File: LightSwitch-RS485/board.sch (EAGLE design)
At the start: 86 parts, among them IC1 PCF8574T, IC2 PCF8574T, K1 OMRON-G3MB-202P-SSR, K2 OMRON-G3MB-202P-SSR, K20 691218410003, K21 691218410003, K22 691218410003, K3 OMRON-G3MB-202P-SSR, K4 OMRON-G3MB-202P-SSR, K5 OMRON-G3MB-202P-SSR, K6 OMRON-G3MB-202P-SSR, K7 OMRON-G3MB-202P-SSR, K8 OMRON-G3MB-202P-SSR, K9 691218410003, T1 BC847, T2 BC847, T3 BC847, T4 BC847, T5 BC847, T6 BC847, T7 BC847, T8 BC847, U1 MAX487ESA+TCBX, U2 ATMEGA328, X1 JST-XH-04-PIN-LONG-PAD, X2 JST-XH-09-PIN-LONG-PAD

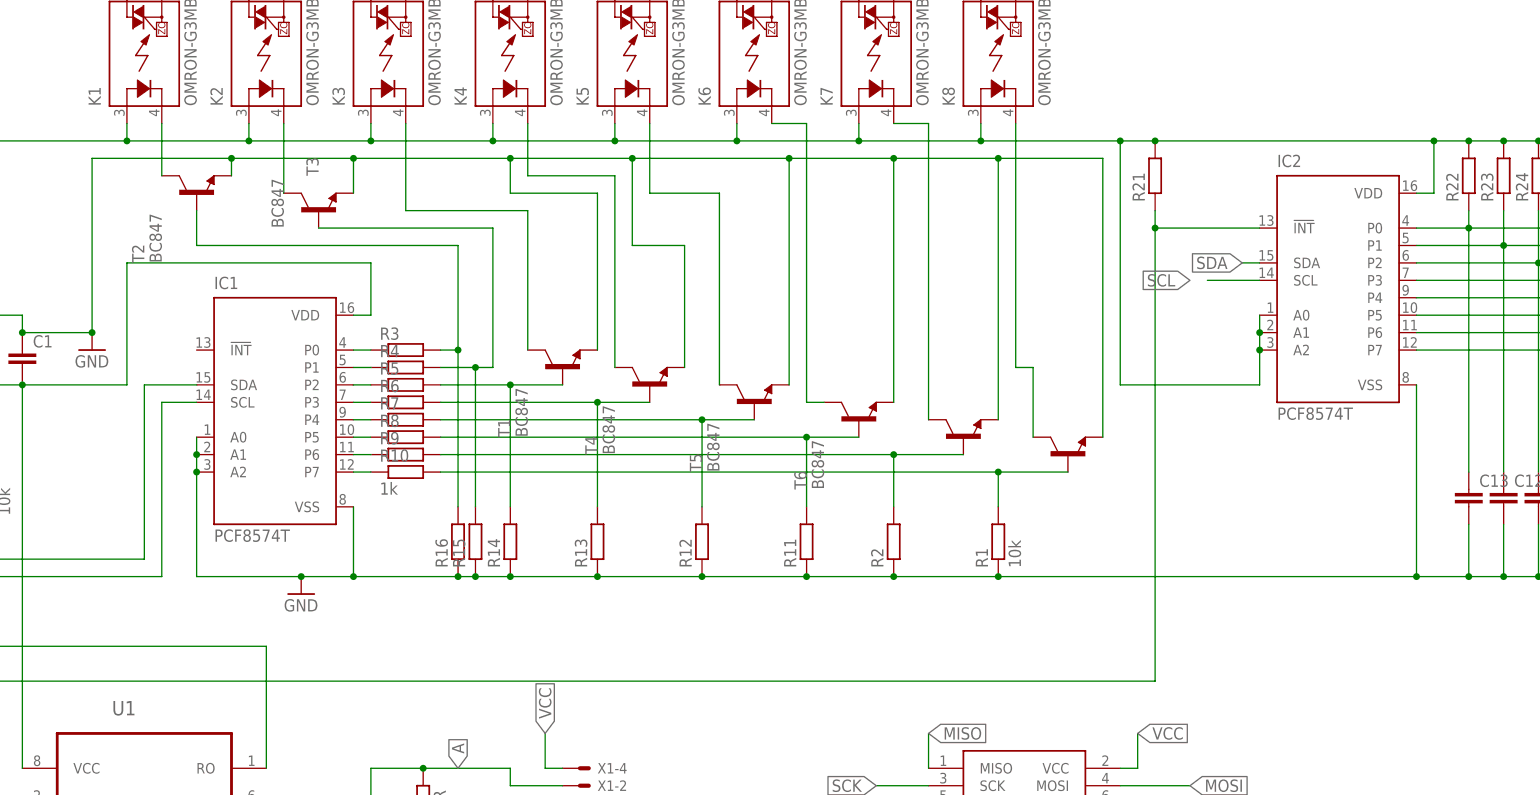
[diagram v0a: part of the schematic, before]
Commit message: fixes
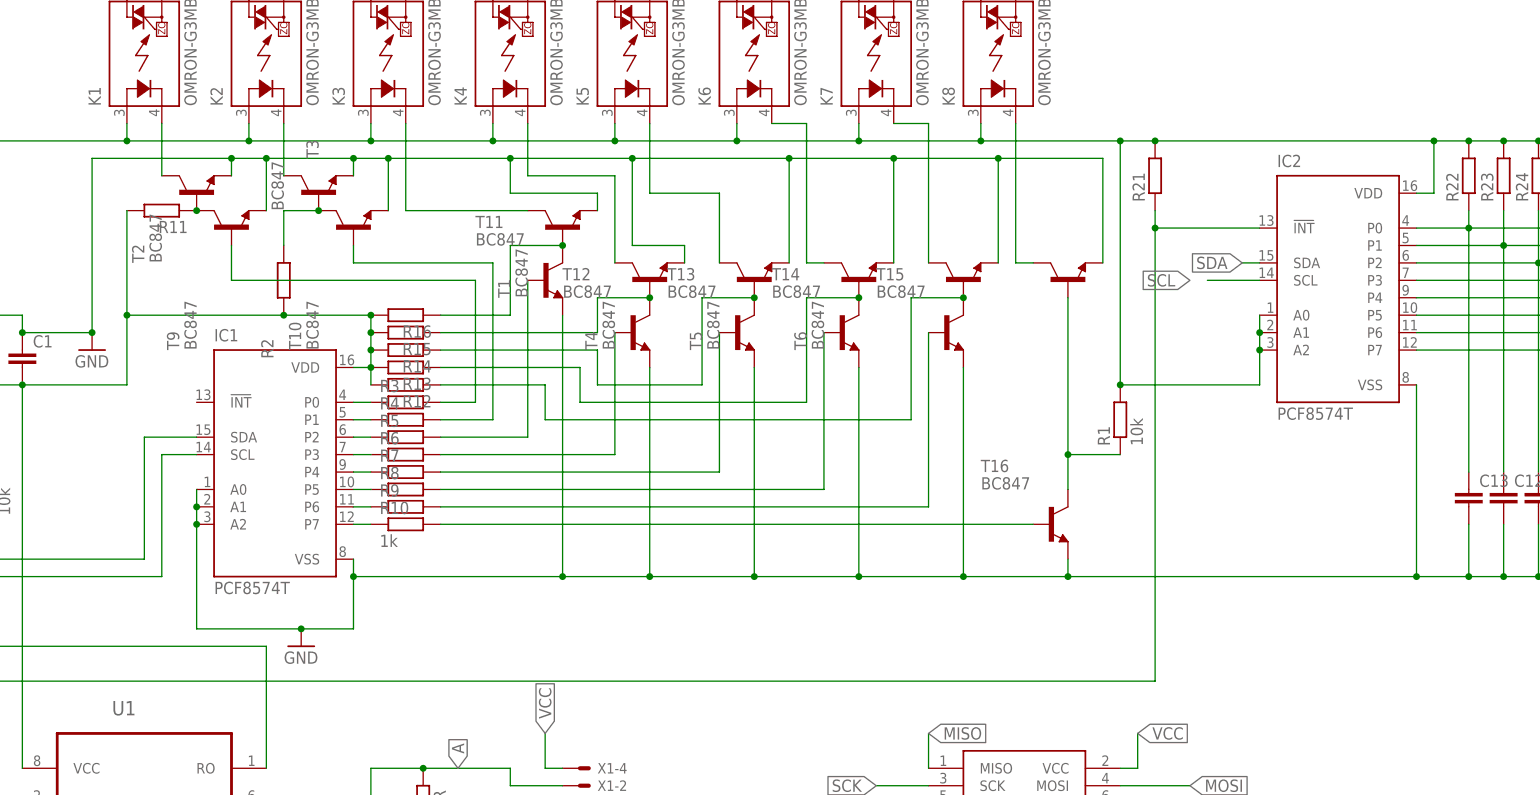
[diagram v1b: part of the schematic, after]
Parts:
- added T10, T11, T12, T13, T14, T15, T16, T9: BC847, nxp_60:BC847
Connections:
- removed net N$2: R1.2, R10.2, T8.B
- new net N$18: R10.2, T16.B
- new net N$51: R12.1, T15.C, T7.B
- new net N$52: R14.1, T13.C, T5.B
- new net N$56: R13.1, T14.C, T6.B
- new net N$67: R5.2, T11.B
- new net N$68: R6.2, T12.B
- new net N$70: R7.2, T13.B
- new net N$73: R8.2, T14.B
- new net N$75: R9.2, T15.B
- net GND: now also T10.E, T11.E, T12.E, T13.E, T14.E, T15.E, T16.E, T9.E; no longer R1.1, R11.1, R12.1, R13.1, R14.1, R15.1, R16.1, R2.1
- net N$5: now also R1.1, T16.C, T8.B; no longer R2.2, R9.2, T7.B
- net N$59: now also R11.1, T9.C; no longer R16.2, R3.2
- net N$61: now also R2.2, T10.C; no longer R15.2, R4.2
- net N$63: now also R3.2, T9.B; no longer R14.2, R5.2, T1.B
- net N$64: now also R4.2, T10.B; no longer R13.2, R6.2, T4.B
- net N$65: now also R16.1, T1.B, T11.C; no longer R12.2, R7.2, T5.B
- net N$66: now also R15.1, T12.C, T4.B; no longer R11.2, R8.2, T6.B
- net VCC: now also R1.2, R11.2, R12.2, R13.2, R14.2, R15.2, R16.2, R2.1
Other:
- moved on the sheet: IC1, R1, R10, R11, R12, R13, R14, R15, R16, R2, R3, R4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
